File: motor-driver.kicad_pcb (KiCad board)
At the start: 4 copper layers, 35 x 27 mm, 108 parts, among them J2 SIGNAL, J3 PWR, J4 RTMI, Q4 SIZ322DT, Q5 SIZ322DT, Q6 SIZ322DT, U1 TMC4671, U2 74LVC3G17, U3 74LVC3G17, U4 TMC6200

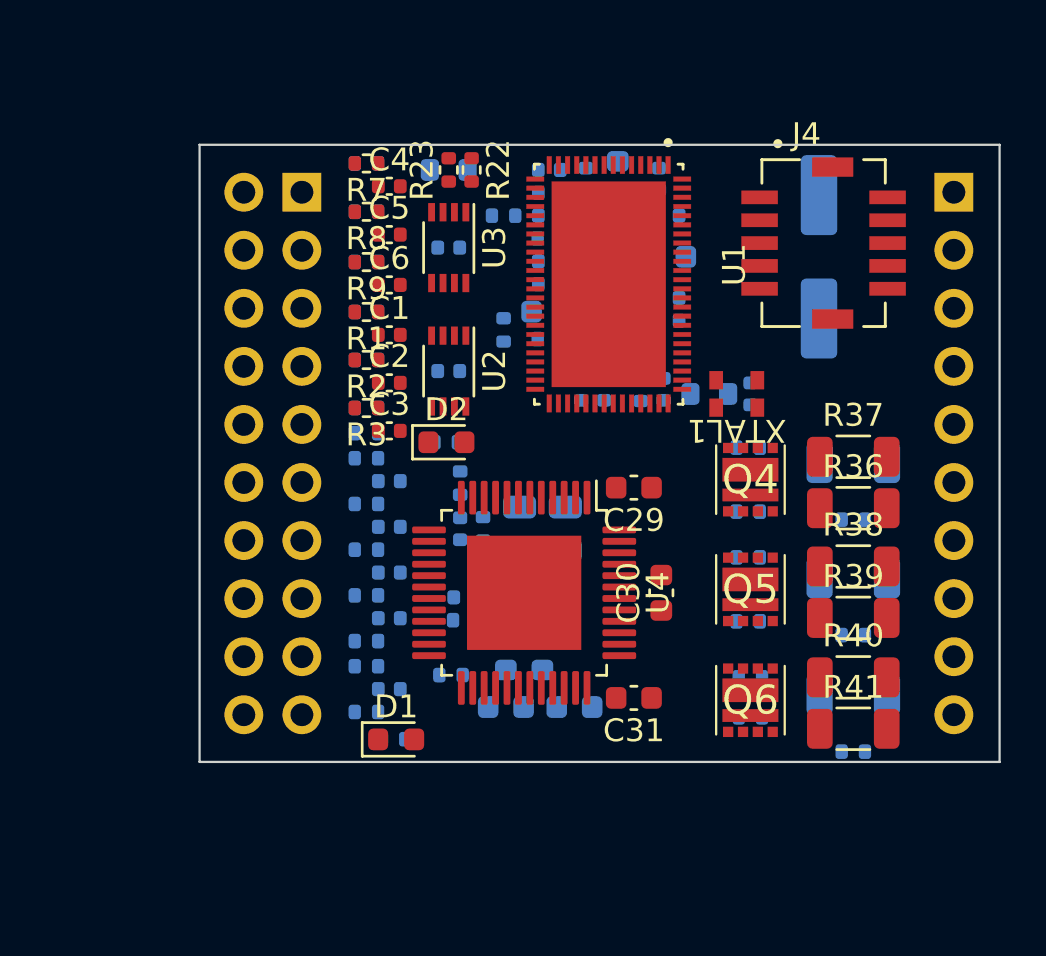
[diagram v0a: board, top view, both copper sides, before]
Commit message: Start routing.
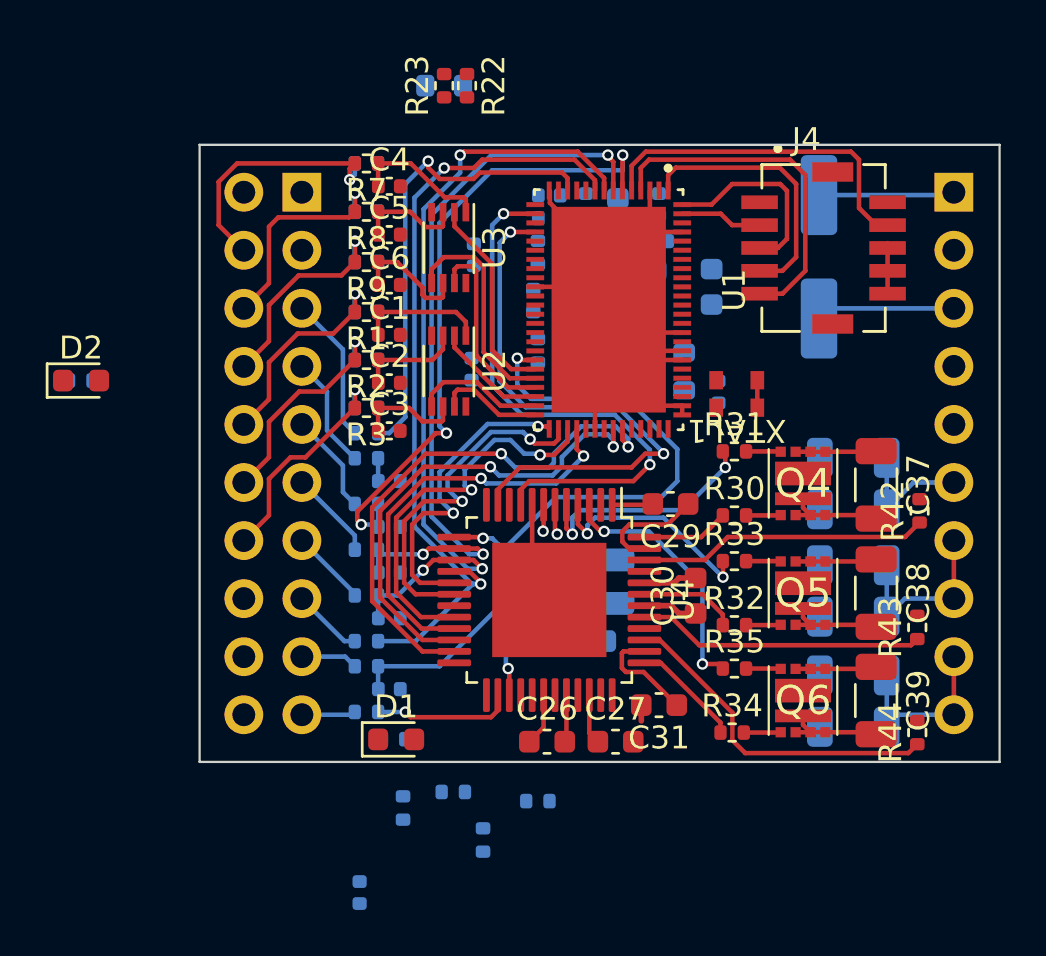
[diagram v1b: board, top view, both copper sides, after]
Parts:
- C26, C27, C37, C38, C39, R30, R31, R32, R33, R34, R35, R42, R43, R44: moved to F.Cu
- R36, R37, R38, R39, R40, R41: moved to B.Cu
- moved C32 16.5 mm to (129.9, 109.0)
- moved R48 16.2 mm to (117.7, 86.6)
- moved D2 16.2 mm to (117.7, 86.6)
- moved R16 13.6 mm to (135.3, 106.7)
- moved R15 13.5 mm to (134.0, 104.6), turned to 180 degrees
- moved R14 8.54 mm to (137.7, 105.0)
- moved C17 7.18 mm to (145.3, 82.5), turned to -90 degrees
- moved R17 6.18 mm to (131.8, 105.3), turned to -90 degrees
- moved R22 3.69 mm to (134.6, 73.7)
- moved R23 3.69 mm to (133.6, 73.7)
- moved TH1 3.69 mm to (133.6, 73.7)
- moved C24 3.26 mm to (141.2, 95.4)
- moved C25 3.26 mm to (139.2, 95.4)
- moved C33 2.94 mm to (137.3, 95.2)
- moved R42 2.93 mm to (154.4, 92.3), turned to 90 degrees
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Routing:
- net /SPI_MISO: track 0.00 -> 34.7 mm, vias 0 -> 2
- net /SPI_MOSI: track 0.00 -> 33.9 mm, vias 0 -> 3
- net /SPI_SCK: track 0.00 -> 32.5 mm, vias 0 -> 3
- net GND: track 0.00 -> 28.5 mm
- net /~{CS_CTRL}: track 0.00 -> 28.3 mm, vias 0 -> 3
- net /Controller/DRV_EN: track 0.00 -> 26.8 mm, vias 0 -> 2
- net /CUR_W: track 0.00 -> 24.9 mm, vias 0 -> 2
- net /CUR_U: track 0.00 -> 24.6 mm, vias 0 -> 2
- net /Controller/WL: track 0.00 -> 23.5 mm, vias 0 -> 2
- net /Controller/WH: track 0.00 -> 21.1 mm, vias 0 -> 2
- net /CTRL_STATUS: track 0.00 -> 20.4 mm, vias 0 -> 1
- net +24V: track 0.00 -> 19.2 mm
- net /Controller/VL: track 0.00 -> 18.1 mm, vias 0 -> 2
- net /Controller/VH: track 0.00 -> 17.2 mm, vias 0 -> 2
- net /Controller/UL: track 0.00 -> 15.8 mm, vias 0 -> 2
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- added copper zone on In1.Cu, net +24V
- added copper zone on In2.Cu, net GND
